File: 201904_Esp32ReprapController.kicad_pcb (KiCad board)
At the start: 2 copper layers, 157.5 x 97.8 mm, 62 parts, among them J1 24V_IN, J10 NOZZLE, J11 BED, J110 MOTOR_X, J12 FAN1, J120 MOTOR_Y, J13 FAN2, J130 MOTOR_Z, J14 FAN3, J140 MOTOR_E, J20 BED_T, J21 NOZZLE_T, J30 Conn_X_Min, J31 Conn_Y_Min, J32 Conn_Z_Min, J40 LCD, J50 SD_Card, J60 BLTouch, Q1 IRLZ44N, Q2 IRLB8743, U1 ESP32-DEVKITC-32D, U2 DcStepDown_LM2596, U3 74HC595, U4 74HC595, U5 ULN2803A

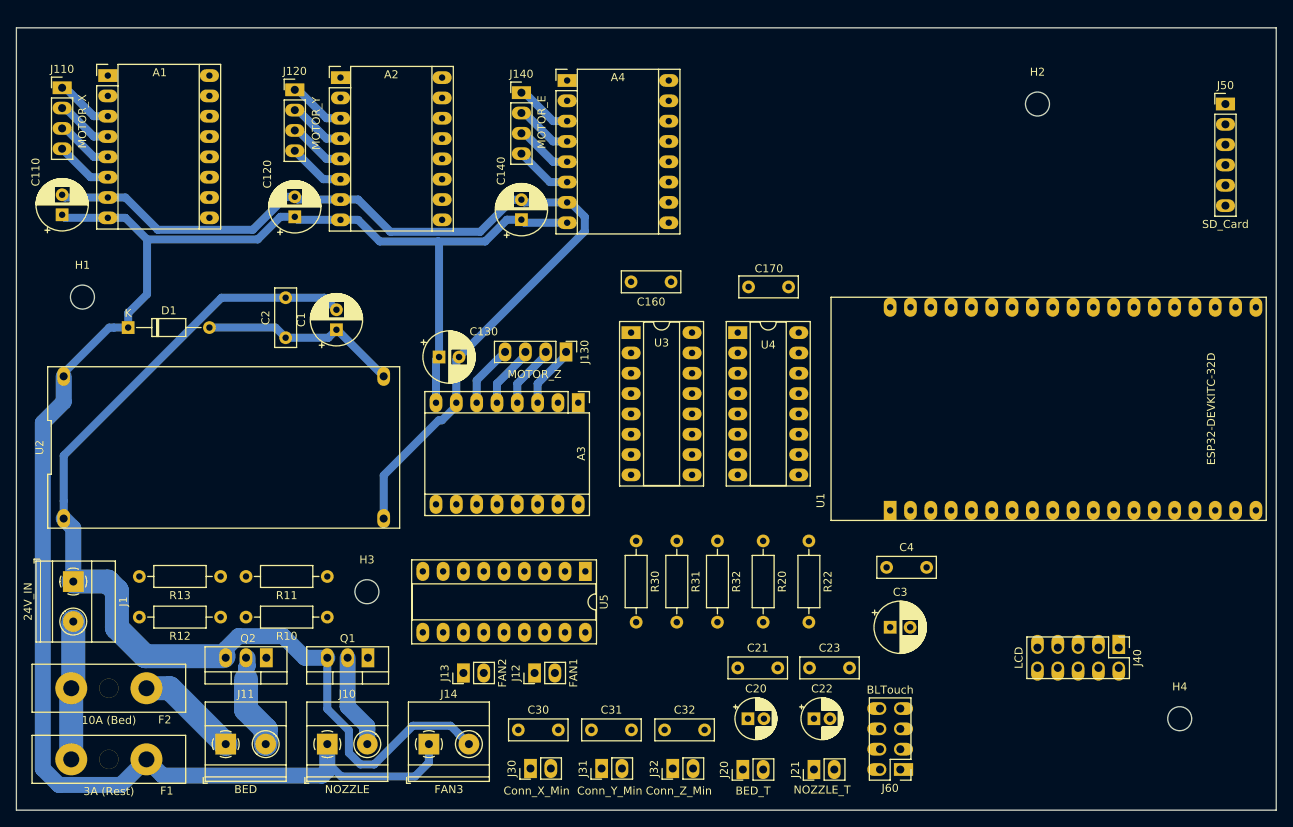
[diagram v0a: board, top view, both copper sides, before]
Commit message: board r3 (milled and built 2019-06)
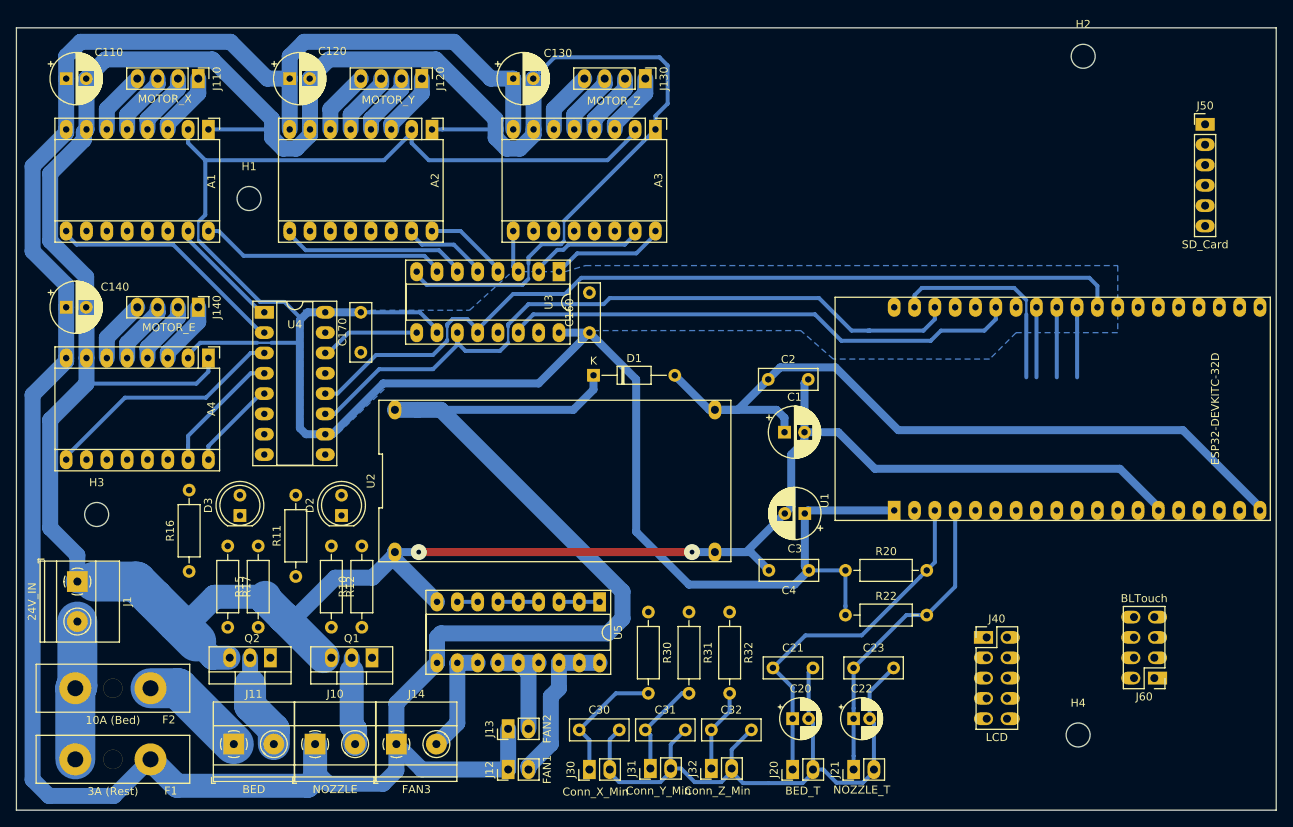
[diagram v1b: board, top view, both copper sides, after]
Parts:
- removed R13: 100k, Felix_Common:R_Axial_DIN0207_L6.3mm_D2.5mm_P10.16mm_Horizontal
- added D2: LED_NOZ, Felix_Common:LED_D5.0mm, F.Cu at (66.0, 90.2)
- added D3: LED_BED, Felix_Common:LED_D5.0mm, F.Cu at (53.3, 90.2)
- added R15: 10, Felix_Common:R_Axial_DIN0207_L6.3mm_D2.5mm_P10.16mm_Horizontal, F.Cu at (55.6, 104.1)
- added R16: 100k, Felix_Common:R_Axial_DIN0207_L6.3mm_D2.5mm_P10.16mm_Horizontal, F.Cu at (47.0, 97.2)
- added R17: 2.2k, Felix_Common:R_Axial_DIN0207_L6.3mm_D2.5mm_P10.16mm_Horizontal, F.Cu at (51.8, 94.0)
- R12: value 10 -> 2.2k
- moved C2 60.5 mm to (119.4, 73.2), turned to 0 degrees
- moved U4 59.2 mm to (56.4, 64.8)
- moved D1 58.5 mm to (97.5, 72.6)
- moved C140 57.9 mm to (31.6, 64.1), turned to 0 degrees
- moved C1 57.5 mm to (121.4, 79.8), turned to 0 degrees
- moved A4 56.7 mm to (49.4, 70.5), turned to 270 degrees
- moved C170 53.6 mm to (68.5, 64.8), turned to 270 degrees
- moved J140 48.5 mm to (48.1, 64.1), turned to 270 degrees
- moved U2 41.6 mm to (92.7, 85.9)
- moved C130 36.0 mm to (87.5, 35.6)
- moved J130 35.6 mm to (104.0, 35.6)
- moved A3 35.5 mm to (105.3, 41.9)
- moved H3 35.1 mm to (35.4, 90.0)
- moved J60 33.7 mm to (167.6, 110.5)
- moved H1 24.2 mm to (54.5, 50.5)
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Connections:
- net /FAN1 renamed /IOx_FAN1
- net /Q132 renamed /Q132_Y_DIR
- net /Q139 renamed /Q139_E_EN
- net /X_MIN renamed /IOx_X_MIN
- net /Y_MIN renamed /IOx_Y_MIN
- A1 pad 15: /Q128 -> /Q137_X_STEP
- A1 pad 16: /Q129 -> /Q135_X_DIR
- A1 pad 9: /Q130 -> /Q138_X_EN
- A2 pad 15: /Q131 -> /Q133_Y_STEP
- A2 pad 9: /Q133 -> /Q134_Y_EN
- A3 pad 15: /Q134 -> /Q130_Z_STEP
- A3 pad 16: /Q135 -> /Q129_Z_DIR
- A3 pad 9: /Q136 -> /Q131_Z_EN
- A4 pad 15: /Q137 -> /Q140_E_STEP
- A4 pad 16: /Q138 -> /Q141_E_DIR
- C20 pad 1: /BED_T -> /I36_T_BED
- C21 pad 1: /BED_T -> /I36_T_BED
- C22 pad 1: /NOZZLE_T -> /I39_T_NOZ
- C23 pad 1: /NOZZLE_T -> /I39_T_NOZ
- C32 pad 1: /Z_MIN -> /IOx_Z_MIN
- J20 pad 1: /BED_T -> /I36_T_BED
- J21 pad 1: /NOZZLE_T -> /I39_T_NOZ
- J32 pad 1: /Z_MIN -> /IOx_Z_MIN
- J40 pad 2: /BTN_ENC -> /IOx_BTN_ENC
- J40 pad 3: /BTN_EN1 -> /IOx_BTN_EN1
- J40 pad 5: /BTN_EN2 -> /IOx_BTN_EN2
- J40 pad 6: /LCD_D4 -> /IOx_LCD_D4
- J40 pad 7: /LCD_RS -> /IOx_LCD_RS
- J40 pad 8: /LCD_EN -> /IOx_LCD_EN
- J60 pad 8: /SERVO -> /IOx_SERVO
- R10 pad 2: /NOZZLE -> /IOx_NOZZLE
- R11 pad 2: /NOZZLE -> /IOx_NOZZLE
- R12 pad 1: Net-(Q2-Pad1) -> Net-(D2-Pad1)
- R12 pad 2: /BED -> Net-(J10-Pad2)
- R20 pad 2: /BED_T -> /I36_T_BED
- R22 pad 2: /NOZZLE_T -> /I39_T_NOZ
- R32 pad 2: /Z_MIN -> /IOx_Z_MIN
- U1 pad 10: /I2S_WS -> /IOx_BTN_ENC
- U1 pad 11: /I2S_DATA -> /IOx_LCD_D4
- U1 pad 12: /BTN_EN2 -> /IOx_LCD_RS
- U1 pad 13: /BTN_EN1 -> /IOx_LCD_EN
- U1 pad 2: /~RESET -> /~ESP32_EN
- U1 pad 22: /LCD_D4 -> /IO21_I2S_BCK
- U1 pad 25: /LCD_EN -> /IO22_I2S_DATA
- U1 pad 3: /NOZZLE_T -> /I36_T_BED
- U1 pad 30: /LCD_RS -> /IO17_I2S_WS
- U1 pad 31: /BEEPER -> Net-(U1-Pad31)
- U1 pad 32: /BED -> /IOx_NOZZLE
- U1 pad 34: /NOZZLE -> /IOx_BED
- U1 pad 35: /Z_MIN -> /IOx_SERVO
- U1 pad 4: /BED_T -> /I39_T_NOZ
- U1 pad 7: /SERVO -> /IOx_Z_MIN
- U1 pad 8: /BTN_ENC -> /IOx_BTN_EN1
- U1 pad 9: /I2S_BCK -> /IOx_BTN_EN2
- U3 pad 1: /Q129 -> /Q129_Z_DIR
- U3 pad 11: /I2S_BCK -> /IO21_I2S_BCK
- U3 pad 12: /I2S_WS -> /IO17_I2S_WS
- U3 pad 14: /I2S_DATA -> /IO22_I2S_DATA
- U3 pad 2: /Q130 -> /Q130_Z_STEP
- U3 pad 3: /Q131 -> /Q131_Z_EN
- U3 pad 5: /Q133 -> /Q133_Y_STEP
- U3 pad 6: /Q134 -> /Q134_Y_EN
- U3 pad 7: /Q135 -> /Q135_X_DIR
- U4 pad 1: /Q137 -> /Q137_X_STEP
- U4 pad 11: /I2S_BCK -> /IO21_I2S_BCK
- U4 pad 12: /I2S_WS -> /IO17_I2S_WS
- U4 pad 2: /Q138 -> /Q138_X_EN
- U4 pad 4: /Q140 -> /Q140_E_STEP
- U4 pad 5: /Q141 -> /Q141_E_DIR
- U4 pad 6: /Q142 -> /Q142_FAN2
- U4 pad 7: /Q143 -> /Q143_FAN3
- U5 pad 4: /Q140 -> /Q142_FAN2
- U5 pad 5: /Q140 -> /Q142_FAN2
- U5 pad 6: /Q140 -> /Q142_FAN2
- U5 pad 7: /Q141 -> /Q143_FAN3
- U5 pad 8: /Q141 -> /Q143_FAN3
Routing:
- net GND: track 253.3 -> 539.9 mm, vias 0 -> 2
- net VCC: track 0.00 -> 267.2 mm
- net +24V: track 224.6 -> 357.7 mm
- net /IO17_I2S_WS: track 0.00 -> 108.3 mm
- net /IO21_I2S_BCK: track 0.00 -> 91.1 mm
- net +5V: track 25.1 -> 95.7 mm
- net /IO22_I2S_DATA: track 0.00 -> 64.9 mm
- net /I36_T_BED: track 0.00 -> 45.9 mm
- net /I39_T_NOZ: track 0.00 -> 39.1 mm
- net /Q135_X_DIR: track 0.00 -> 30.9 mm
- net /Q139_E_EN: track 0.00 -> 30.5 mm
- net /Q138_X_EN: track 0.00 -> 30.3 mm
- net /SD_MOSI: track 0.00 -> 26.1 mm
- net /Q134_Y_EN: track 0.00 -> 23.5 mm
- net Net-(J12-Pad2): track 0.00 -> 20.0 mm
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- added copper zone on B.Cu, net GND
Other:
- net class Default: trace_width 0.3 -> 0.5; via_dia 0.8 -> 2; via_drill 0.4 -> 0.6
